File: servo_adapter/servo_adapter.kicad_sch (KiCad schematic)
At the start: 16 parts, among them J1 T4140012081-000, J2 Conn_01x10_Socket, J3 Conn_01x02_Socket, Q1 MUN5233, Q2 MUN5233, Q3 MUN5233, Q4 MUN5233

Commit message: Added footprints for Caps, mounting holes and 2.54mm servo connector.
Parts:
- C1: footprint (none) -> Capacitor_SMD:C_0805_2012Metric
- H1, H2: footprint (none) -> MountingHole:MountingHole_2.7mm_M2.5
- J2: footprint (none) -> Connector_PinSocket_2.54mm:PinSocket_1x10_P2.54mm_Vertical
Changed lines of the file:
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@@
 			)
 		)
-		(property "Footprint" ""
+		(property "Footprint" "Capacitor_SMD:C_0805_2012Metric"
 			(at 229.5652 78.74 0)
 			(effects
@@
 			)
 		)
-		(property "Footprint" ""
+		(property "Footprint" "MountingHole:MountingHole_2.7mm_M2.5"
 			(at 228.6 110.49 0)
 			(effects
@@
 			)
 		)
-		(property "Footprint" ""
+		(property "Footprint" "Connector_PinSocket_2.54mm:PinSocket_1x10_P2.54mm_Vertical"
 			(at 266.7 60.96 0)
 			(effects
@@
 			)
 		)
-		(property "Footprint" ""
+		(property "Footprint" "MountingHole:MountingHole_2.7mm_M2.5"
 			(at 228.6 125.73 0)
 			(effects

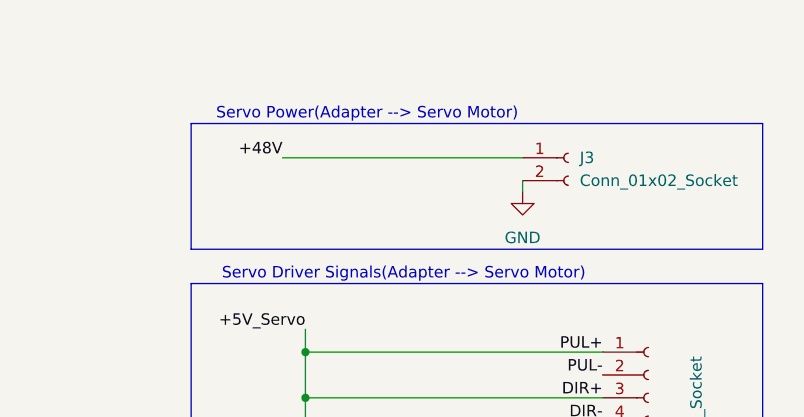
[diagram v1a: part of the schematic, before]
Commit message: Removed old placeholder connector for the TL4141012051-000.
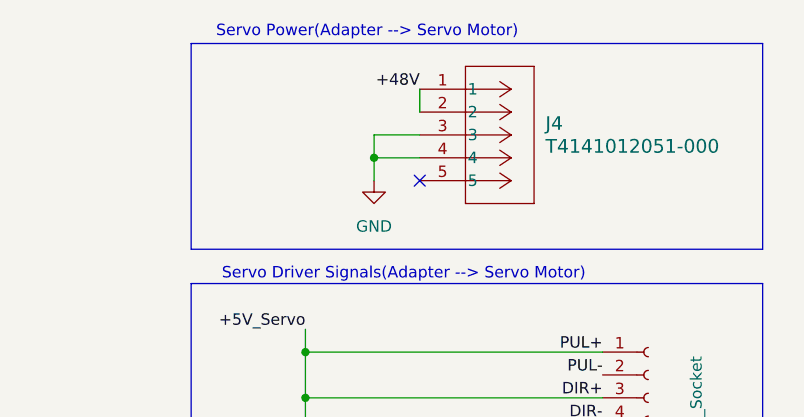
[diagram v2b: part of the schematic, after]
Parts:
- removed J3: Conn_01x02_Socket, symbol Connector:Conn_01x02_Socket
- added J4: T4141012051-000, servo_adapter_fp:CONN5_T4141012051, symbol T4141L12051-000:T4141012051-000
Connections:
- net +48V: now also J4.1, J4.2
- net GND: now also J4.3, J4.4
- no-connect marks 0 -> 1
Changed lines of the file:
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@@
 	)
 	(rectangle
-		(start 215.9 25.4)
+		(start 215.9 16.51)
 		(end 279.4 39.37)
 		(stroke
@@
 	(text "Servo Power(Adapter --> Servo Motor)"
 		(exclude_from_sim no)
-		(at 235.458 24.384 0)
+		(at 235.458 15.24 0)
 		(effects
 			(font
@@
 	)
 	(junction
+		(at 236.22 29.21)
+		(diameter 0)
+		(color 0 0 0 0)
+	)
+	(junction
 		(at 228.6 55.88)
 		(diameter 0)
@@
 		(color 0 0 0 0)
 	)
+	(no_connect
+		(at 241.3 31.75)
+	)
 	(wire
 		(pts
@@
 	(wire
 		(pts
+			(xy 236.22 26.67) (xy 236.22 29.21)
+		)
+		(stroke
+			(width 0)
+			(type default)
+		)
+	)
+	(wire
+		(pts
 			(xy 228.6 78.74) (xy 228.6 86.36)
 		)
@@
 	(wire
 		(pts
-			(xy 252.73 29.21) (xy 226.06 29.21)
+			(xy 241.3 26.67) (xy 236.22 26.67)
 		)
 		(stroke
@@
 	(wire
 		(pts
-			(xy 252.73 31.75) (xy 252.73 33.02)
+			(xy 241.3 29.21) (xy 236.22 29.21)
 		)
 		(stroke
@@
 	(wire
 		(pts
+			(xy 241.3 21.59) (xy 241.3 24.13)
+		)
+		(stroke
+			(width 0)
+			(type default)
+		)
+	)
+	(wire
+		(pts
 			(xy 228.6 60.96) (xy 228.6 55.88)
 		)
@@
 		(pts
 			(xy 228.6 71.12) (xy 228.6 66.04)
+		)
+		(stroke
+			(width 0)
+			(type default)
+		)
+	)
+	(wire
+		(pts
+			(xy 236.22 29.21) (xy 236.22 31.75)
 		)
 		(stroke
@@
 		)
 	)
-	(label "+48V"
-		(at 226.06 29.21 180)
-		(effects
-			(font
-				(size 1.27 1.27)
-			)
-			(justify right bottom)
-		)
-	)
 	(label "PED-"
 		(at 261.62 68.58 180)
@@
 	(label "PED_OUT"
 		(at 92.71 25.4 180)
+		(effects
+			(font
+				(size 1.27 1.27)
+			)
+			(justify right bottom)
+		)
+	)
+	(label "+48V"
+		(at 241.3 21.59 180)
 		(effects
 			(font
@@
 	)
 	(symbol
-		(lib_id "Connector:Conn_01x02_Socket")
-		(at 257.81 29.21 0)
+		(lib_id "T4141L12051-000:T4141012051-000")
+		(at 241.3 21.59 0)
 		(unit 1)
 		(exclude_from_sim no)
@@
 		(dnp no)
 		(fields_autoplaced yes)
-		(property "Reference" "J3"
-			(at 259.08 29.2099 0)
-			(effects
-				(font
-					(size 1.27 1.27)
+		(property "Reference" "J4"
+			(at 255.27 25.3999 0)
+			(effects
+				(font
+					(size 1.524 1.524)
 				)
 				(justify left)
 			)
 		)
-		(property "Value" "Conn_01x02_Socket"
-			(at 259.08 31.7499 0)
-			(effects
-				(font
-					(size 1.27 1.27)
+		(property "Value" "T4141012051-000"
+			(at 255.27 27.9399 0)
+			(effects
+				(font
+					(size 1.524 1.524)
 				)
 				(justify left)
 			)
 		)
-		(property "Footprint" ""
-			(at 257.81 29.21 0)
-			(effects
-				(font
-					(size 1.27 1.27)
-				)
-				(hide yes)
-			)
-		)
-		(property "Datasheet" "~"
-			(at 257.81 29.21 0)
-			(effects
-				(font
-					(size 1.27 1.27)
-				)
-				(hide yes)
-			)
-		)
-		(property "Description" "Generic connector, single row, 01x02, script generated"
-			(at 257.81 29.21 0)
-			(effects
-				(font
-					(size 1.27 1.27)
-				)
-				(hide yes)
-			)
+		(property "Footprint" "servo_adapter_fp:CONN5_T4141012051"
+			(at 241.3 21.59 0)
+			(effects
+				(font
+					(size 1.27 1.27)
+					(italic yes)
+				)
+				(hide yes)
+			)
+		)
+		(property "Datasheet" "T4141012051-000"
+			(at 241.3 21.59 0)
+			(effects
+				(font
+					(size 1.27 1.27)
+					(italic yes)
+				)
+				(hide yes)
+			)
+		)
+		(property "Description" ""
+			(at 241.3 21.59 0)
+			(effects
+				(font
+					(size 1.27 1.27)
+				)
+				(hide yes)
+			)
+		)
+		(pin "3"
+		)
+		(pin "4"
 		)
 		(pin "2"
 		)
 		(pin "1"
+		)
+		(pin "5"
 		)
 		(instances
 			(project ""
 				(path "/d2a6932a-1682-4170-bbbb-2fb2c0f935d7"
-					(reference "J3")
+					(reference "J4")
 					(unit 1)
 				)
@@
 	)
 	(symbol
-		(lib_id "power:GND")
-		(at 252.73 33.02 0)
-		(unit 1)
-		(exclude_from_sim no)
-		(in_bom yes)
-		(on_board yes)
-		(dnp no)
-		(fields_autoplaced yes)
-		(property "Reference" "#PWR04"
-			(at 252.73 39.37 0)
-			(effects
-				(font
-					(size 1.27 1.27)
-				)
-				(hide yes)
-			)
-		)
-		(property "Value" "GND"
-			(at 252.73 38.1 0)
-			(effects
-				(font
-					(size 1.27 1.27)
-				)
-			)
-		)
-		(property "Footprint" ""
-			(at 252.73 33.02 0)
-			(effects
-				(font
-					(size 1.27 1.27)
-				)
-				(hide yes)
-			)
-		)
-		(property "Datasheet" ""
-			(at 252.73 33.02 0)
-			(effects
-				(font
-					(size 1.27 1.27)
-				)
-				(hide yes)
-			)
-		)
-		(property "Description" "Power symbol creates a global label with name \"GND\" , ground"
-			(at 252.73 33.02 0)
-			(effects
-				(font
-					(size 1.27 1.27)
-				)
-				(hide yes)
-			)
-		)
-		(pin "1"
-		)
-		(instances
-			(project "servo_adapter"
-				(path "/d2a6932a-1682-4170-bbbb-2fb2c0f935d7"
-					(reference "#PWR04")
-					(unit 1)
-				)
-			)
-		)
-	)
-	(symbol
 		(lib_id "PCM_Transistor_BJT_Pre-Biased_AKL:MUN5233")
 		(at 35.56 138.43 0)
@@
 					(unit 1)
 				)
+			)
+		)
+	)
+	(symbol
+		(lib_id "power:GND")
+		(at 236.22 31.75 0)
+		(unit 1)
+		(exclude_from_sim no)
+		(in_bom yes)
+		(on_board yes)
+		(dnp no)
+		(fields_autoplaced yes)
+		(property "Reference" "#PWR08"
+			(at 236.22 38.1 0)
+			(effects
+				(font
+					(size 1.27 1.27)
+				)
+				(hide yes)
+			)
+		)
+		(property "Value" "GND"
+			(at 236.22 36.83 0)
+			(effects
+				(font
+					(size 1.27 1.27)
+				)
+			)
+		)
+		(property "Footprint" ""
+			(at 236.22 31.75 0)
+			(effects
+				(font
+					(size 1.27 1.27)
+				)
+				(hide yes)
+			)
+		)
+		(property "Datasheet" ""
+			(at 236.22 31.75 0)
+			(effects
+				(font
+					(size 1.27 1.27)
+				)
+				(hide yes)
+			)
+		)
+		(property "Description" "Power symbol creates a global label with name \"GND\" , ground"
+			(at 236.22 31.75 0)
+			(effects
+				(font
+					(size 1.27 1.27)
+				)
+				(hide yes)
+			)
+		)
+		(pin "1"
+		)
+		(instances
+			(project "servo_adapter"
+				(path "/d2a6932a-1682-4170-bbbb-2fb2c0f935d7"
+					(reference "#PWR08")
+					(unit 1)
+				)
